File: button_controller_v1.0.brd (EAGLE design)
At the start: 100 x 44.1 mm, 88 parts, among them IC2 4051D, IC3 4520D, IC5 4051D

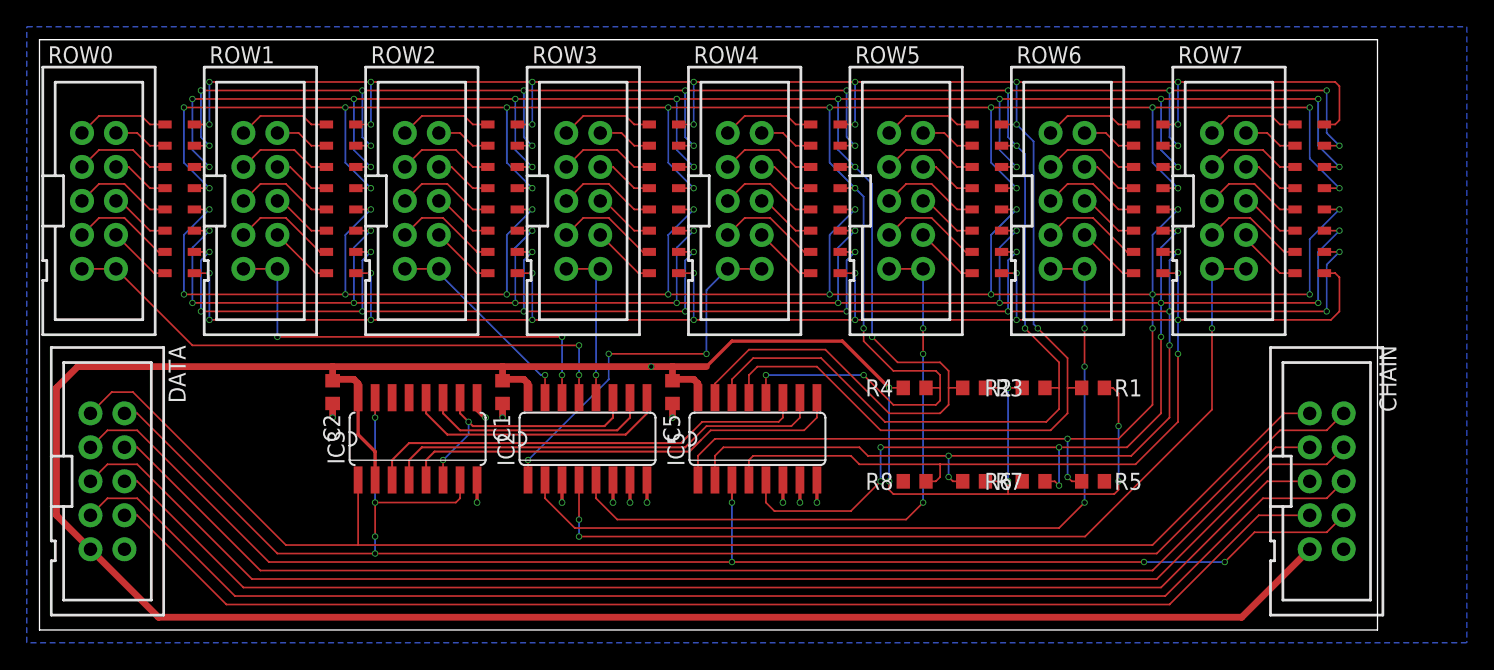
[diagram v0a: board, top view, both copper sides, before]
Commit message: As small as it gets
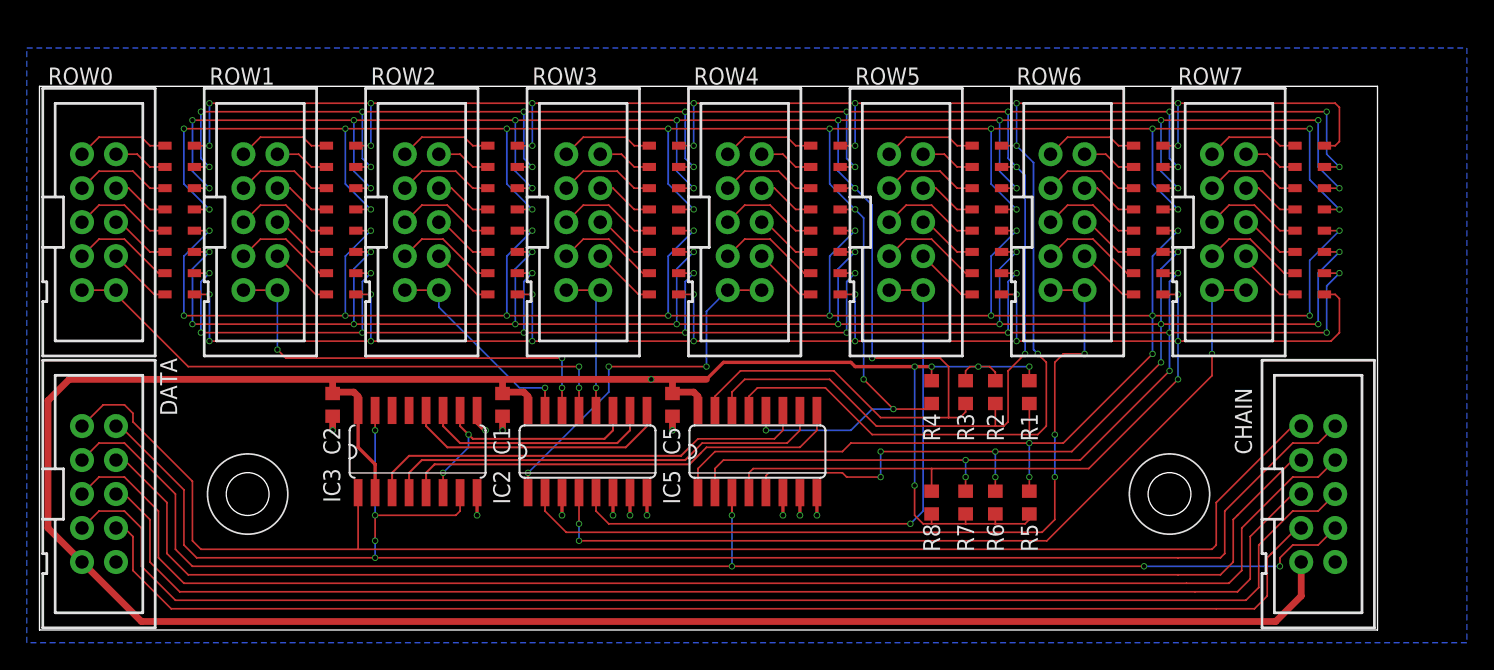
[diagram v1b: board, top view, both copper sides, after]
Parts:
- moved R5 5.02 mm to (74.0, 9.53), turned to 270 degrees
- moved R1 4.77 mm to (74.0, 17.8), turned to 90 degrees
- moved R6 3.27 mm to (71.4, 9.53), turned to 270 degrees
- moved R2 2.88 mm to (71.4, 17.8), turned to 90 degrees
- moved R8 2.03 mm to (66.7, 9.53), turned to 270 degrees
- moved R7 1.71 mm to (69.2, 9.53), turned to 270 degrees
- moved D12 1.59 mm to (10.5, 31.4)
- moved D13 1.59 mm to (10.5, 29.8)
- moved D16 1.59 mm to (10.5, 25.1)
- moved D20 1.59 mm to (34.6, 31.4)
- moved D21 1.59 mm to (34.6, 29.8)
- moved D24 1.59 mm to (34.6, 25.1)
- moved D28 1.59 mm to (22.5, 31.4)
- moved D29 1.59 mm to (22.5, 29.8)
- moved D32 1.59 mm to (22.5, 25.1)
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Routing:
- net +5V: track 239.6 -> 231.9 mm, vias 7 -> 6
- net COL5: track 189.1 -> 182.3 mm
- net COL3: track 185.2 -> 178.8 mm
- net COL1: track 179.3 -> 173.9 mm
- net COL6: track 179.8 -> 175.6 mm
- net COL7: track 167.3 -> 163.2 mm
- net COL4: track 200.0 -> 196.3 mm
- net CLK: track 105.5 -> 109.1 mm
- net ROW7: track 68.5 -> 64.9 mm
- net BUTTON_VAL_CHAIN_1: track 96.2 -> 99.8 mm
- net BUTTON_VAL_CHAIN_2: track 101.8 -> 105.2 mm
- net BUTTON_VAL_CHAIN_3: track 95.2 -> 98.4 mm
- net RESET: track 119.3 -> 122.4 mm
- net COL0: track 172.4 -> 169.4 mm
- net BUTTON_VAL_CHAIN_4: track 100.8 -> 103.8 mm
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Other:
- board size 100 x 44.1 mm -> 100 x 40.6 mm
